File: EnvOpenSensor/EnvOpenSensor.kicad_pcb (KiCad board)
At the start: 2 copper layers, 89.7 x 67.5 mm, 31 parts, among them J1 USB_C_Receptacle_USB2.0_16P, J2 AVR-ISP-6, SW1 SW_Push, SW2 SW_Push, SW3 SW_Push, SW4 SW_Push, U1 SCD41-D-R2, U2 Si7021-A20, U3 SPX3819M5-L-3-3, U4 ATtiny85-20S

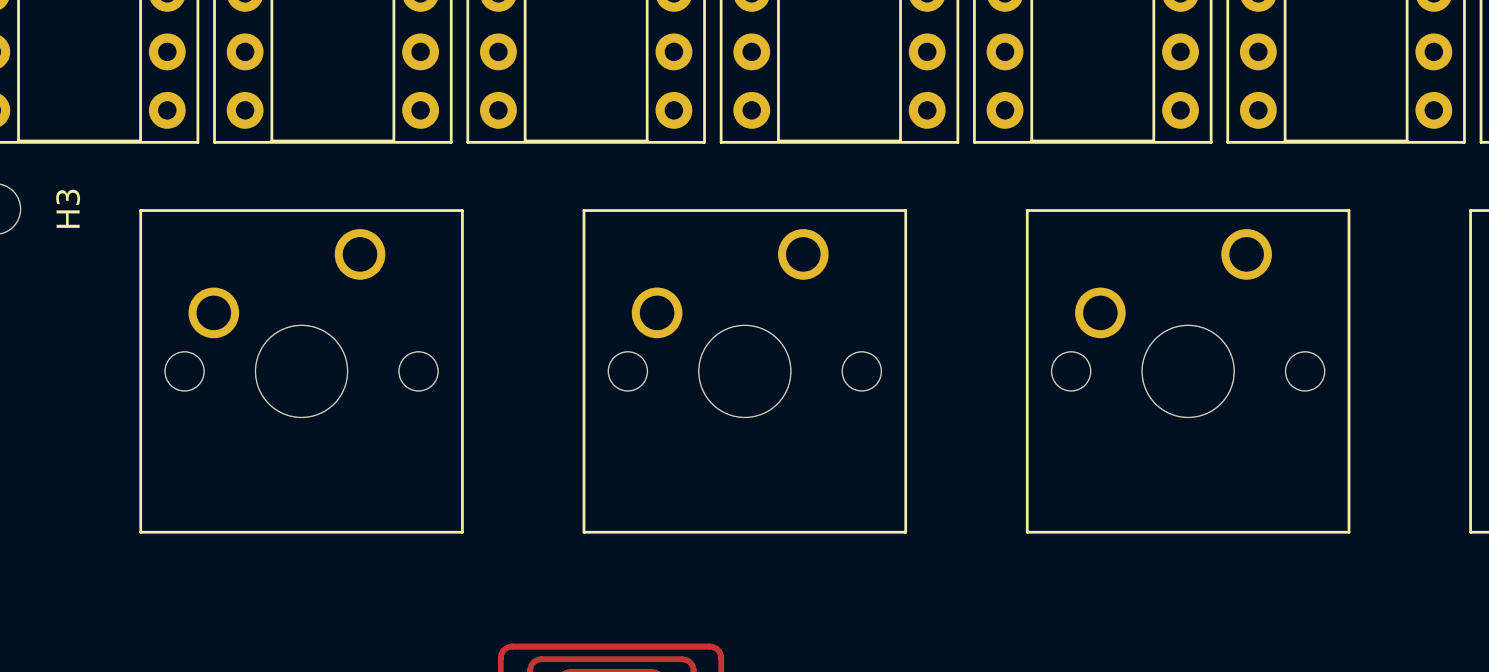
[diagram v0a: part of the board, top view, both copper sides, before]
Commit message: forgot some stuff
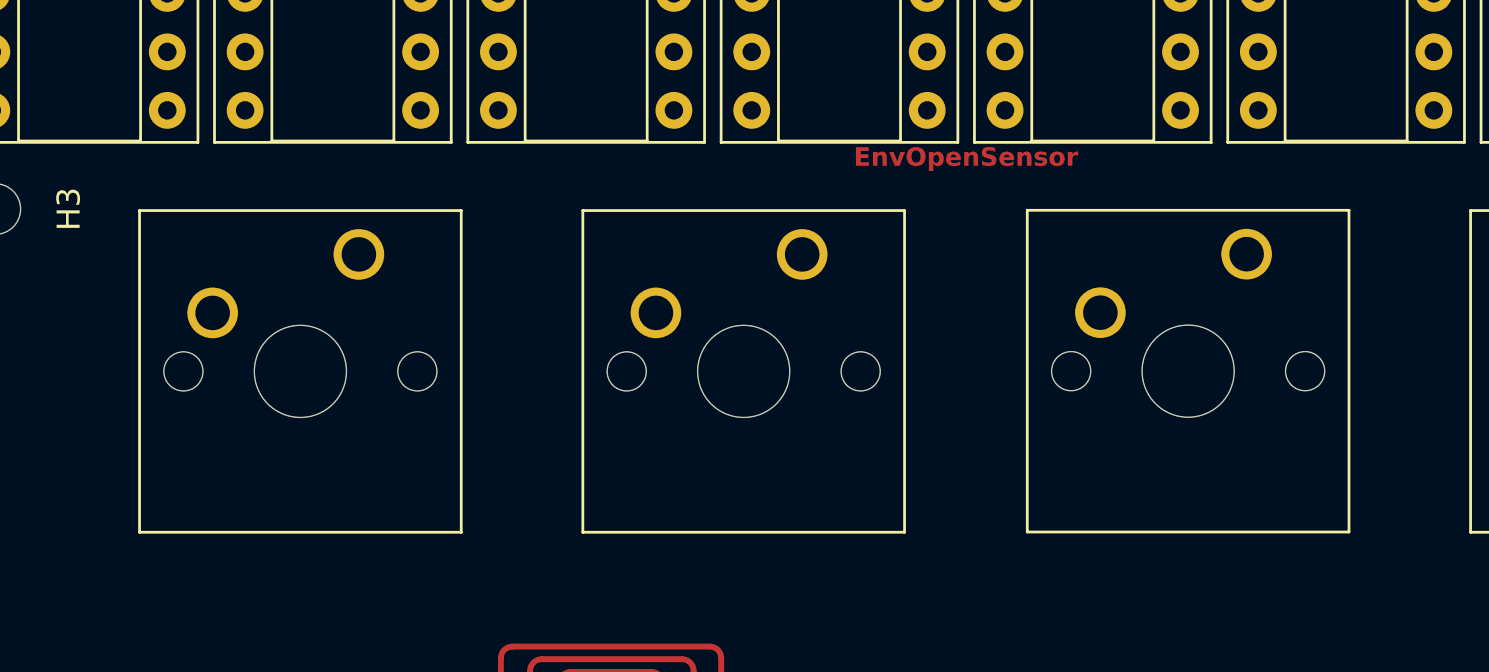
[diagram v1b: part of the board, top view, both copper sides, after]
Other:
- board text added: "EnvOpenSensor"
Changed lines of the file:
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@@
   )
   (footprint "Button_Switch_Keyboard:SW_Cherry_MX_1.00u_PCB" (layer "F.Cu")
-    (at 71.94 36.12)
+    (at 71.94 36.11)
     (descr "Cherry MX keyswitch, 1.00u, PCB mount, http://cherryamericas.com/wp-content/uploads/2014/12/mx_cat.pdf")
     (tags "Cherry MX keyswitch 1.00u PCB")
@@
   )
   (footprint "Button_Switch_Keyboard:SW_Cherry_MX_1.00u_PCB" (layer "F.Cu")
-    (at 33.44 36.12)
+    (at 33.39 36.12)
     (descr "Cherry MX keyswitch, 1.00u, PCB mount, http://cherryamericas.com/wp-content/uploads/2014/12/mx_cat.pdf")
     (tags "Cherry MX keyswitch 1.00u PCB")
@@
   )
   (footprint "Button_Switch_Keyboard:SW_Cherry_MX_1.00u_PCB" (layer "F.Cu")
-    (at 52.69 36.12)
+    (at 52.64 36.12)
     (descr "Cherry MX keyswitch, 1.00u, PCB mount, http://cherryamericas.com/wp-content/uploads/2014/12/mx_cat.pdf")
     (tags "Cherry MX keyswitch 1.00u PCB")
@@
   (gr_line (start 15 77.5) (end 15 15)
     (stroke (width 0.1) (type default)) (layer "Edge.Cuts"))
+  (gr_text "EnvOpenSensor" (at 59.75 31.9) (layer "F.Cu")
+    (effects (font (size 0.8 0.8) (thickness 0.15) bold))
+  )
   (gr_text "env" (at 59.825 70) (layer "F.Mask")
     (effects (font (face "Dissolve Regular") (size 5 5) (thickness 0.15)))
